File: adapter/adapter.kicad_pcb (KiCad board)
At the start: 2 copper layers, 41.8 x 50.8 mm, 29 parts, among them J1 Serial, J2 Ribbon, J3 RGB, J4 Ribbon, J5 Battery charge, SW1 SW_SPST, U1 Dual MCU: RP2040 + nice!nano, U2 AP1603WG-7

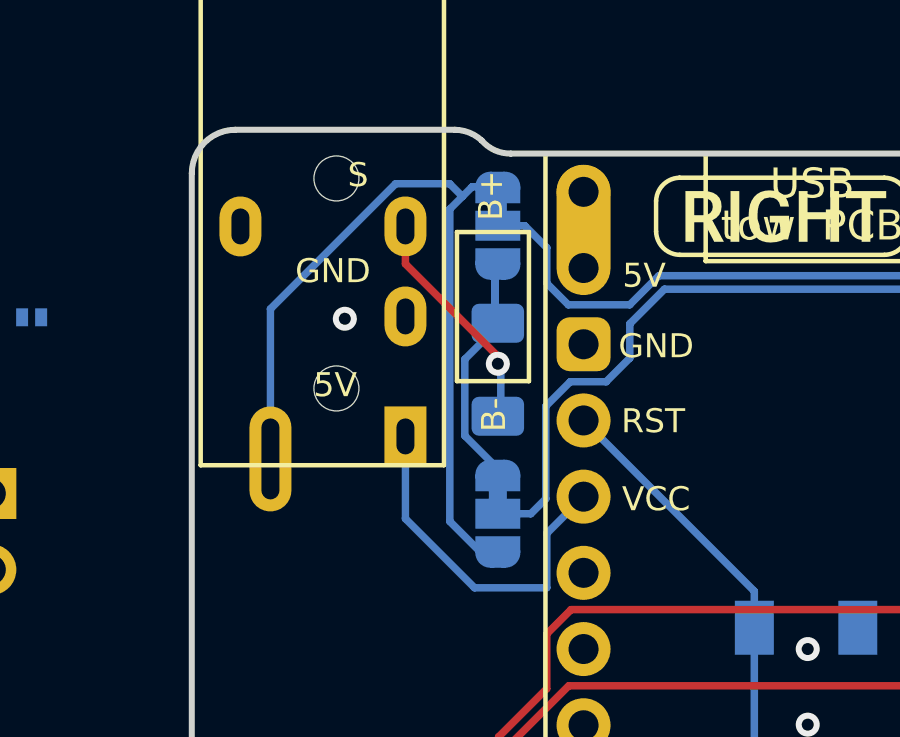
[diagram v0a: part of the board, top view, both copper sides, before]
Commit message: pcb: fix up drc
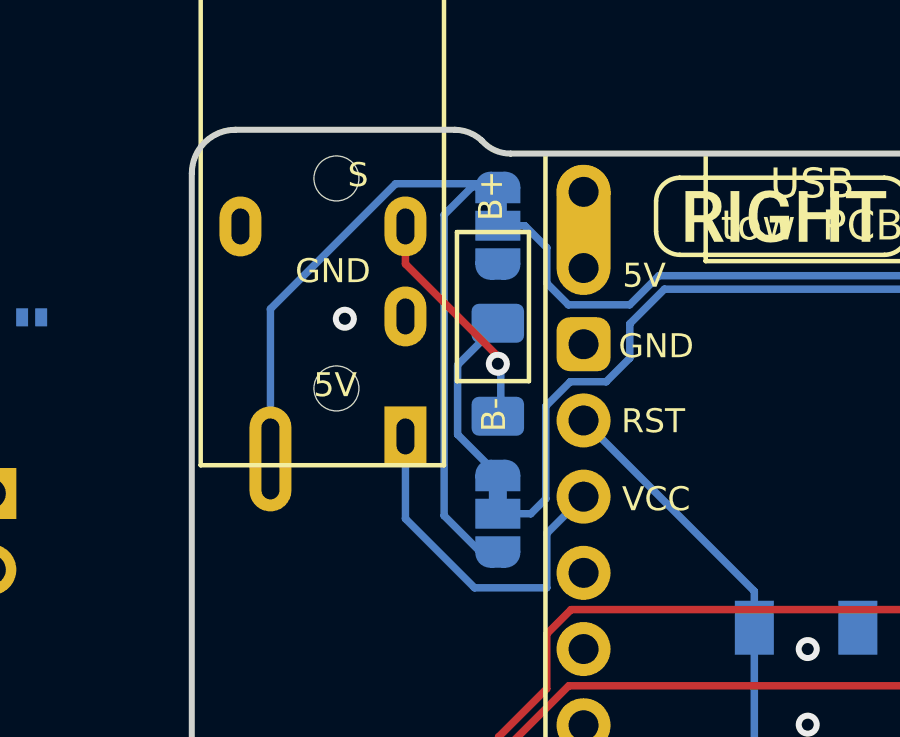
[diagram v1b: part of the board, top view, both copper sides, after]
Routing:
- net serial_l: track 10.0 -> 6.42 mm
- net TX_L: track 27.8 -> 29.1 mm
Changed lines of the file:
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@@
 	)
 	(segment
-		(start 126.6 74.85)
-		(end 126.6 77.4)
+		(start 126.36 75.04)
+		(end 126.36 77.36)
 		(width 0.25)
 		(layer "B.Cu")
@@
 	)
 	(segment
-		(start 127.6 73.45)
-		(end 127.8 73.65)
+		(start 127.918198 73.481802)
+		(end 126.36 75.04)
 		(width 0.25)
 		(layer "B.Cu")
@@
 	)
 	(segment
-		(start 127.6 71.7)
-		(end 127.6 73.45)
-		(width 0.25)
-		(layer "B.Cu")
-		(net 14)
-	)
-	(segment
-		(start 127.6 71.7)
-		(end 127.6 73.163604)
-		(width 0.25)
-		(layer "B.Cu")
-		(net 14)
-	)
-	(segment
-		(start 126.6 77.4)
-		(end 127.9 78.7)
-		(width 0.25)
-		(layer "B.Cu")
-		(net 14)
-	)
-	(segment
-		(start 127.6 73.163604)
-		(end 127.918198 73.481802)
-		(width 0.25)
-		(layer "B.Cu")
-		(net 14)
-	)
-	(segment
-		(start 127.8 73.65)
-		(end 126.6 74.85)
+		(start 126.36 77.36)
+		(end 127.7 78.7)
 		(width 0.25)
 		(layer "B.Cu")
@@
 	)
 	(segment
-		(start 126.1 69.845)
-		(end 126.1 80.255)
-		(width 0.25)
-		(layer "B.Cu")
-		(net 33)
-	)
-	(segment
-		(start 126.095 69)
-		(end 126.52 69.425)
+		(start 126.845 69.1)
+		(end 127.7 69.1)
 		(width 0.25)
 		(layer "B.Cu")
@@
 	)
 	(segment
-		(start 126.1 80.255)
-		(end 127.145 81.3)
-		(width 0.25)
-		(layer "B.Cu")
-		(net 33)
-	)
-	(segment
-		(start 127.6 69.1)
-		(end 126.845 69.1)
+		(start 124.293169 69)
+		(end 127.6 69)
 		(width 0.25)
 		(layer "B.Cu")
@@
 	)
 	(segment
-		(start 126.845 69.1)
-		(end 126.52 69.425)
+		(start 125.91 80.065)
+		(end 127.145 81.3)
 		(width 0.25)
 		(layer "B.Cu")
@@
 	)
 	(segment
-		(start 124.293169 69)
-		(end 126.095 69)
+		(start 125.91 70.035)
+		(end 125.91 80.065)
 		(width 0.25)
 		(layer "B.Cu")
@@
 	)
 	(segment
-		(start 126.52 69.425)
-		(end 126.1 69.845)
-		(width 0.25)
-		(layer "B.Cu")
+		(start 127.6 69)
+		(end 127.7 69.1)
+		(width 0.25)
+		(layer "B.Cu")
+		(net 33)
+	)
+	(segment
+		(start 125.91 70.035)
+		(end 126.845 69.1)
+		(width 0.25)
+		(layer "B.Cu")
